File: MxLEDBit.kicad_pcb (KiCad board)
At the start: 2 copper layers, 94 x 91.4 mm, 355 parts, among them P11 CONN_01X01, P12 CONN_01X01, P13 CONN_01X01, P14 CONN_01X01, P15 CONN_01X01, P16 CONN_01X01, P2 CONN_01X01, P21 CONN_01X01, P22 CONN_01X01, P23 CONN_01X01, P24 CONN_01X01, SW1 SW_PUSH, U1 SK6812mini, U2 ProMicro

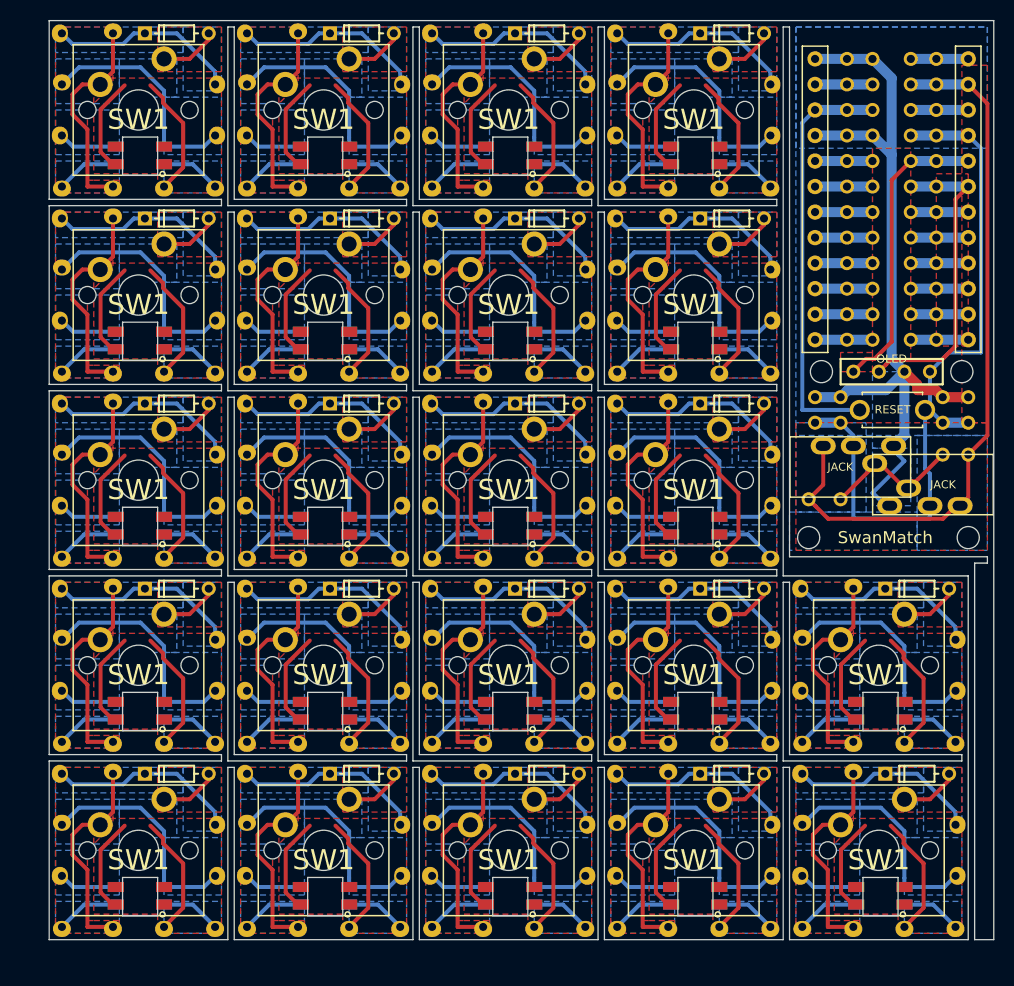
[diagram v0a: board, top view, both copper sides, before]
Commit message: second ordered
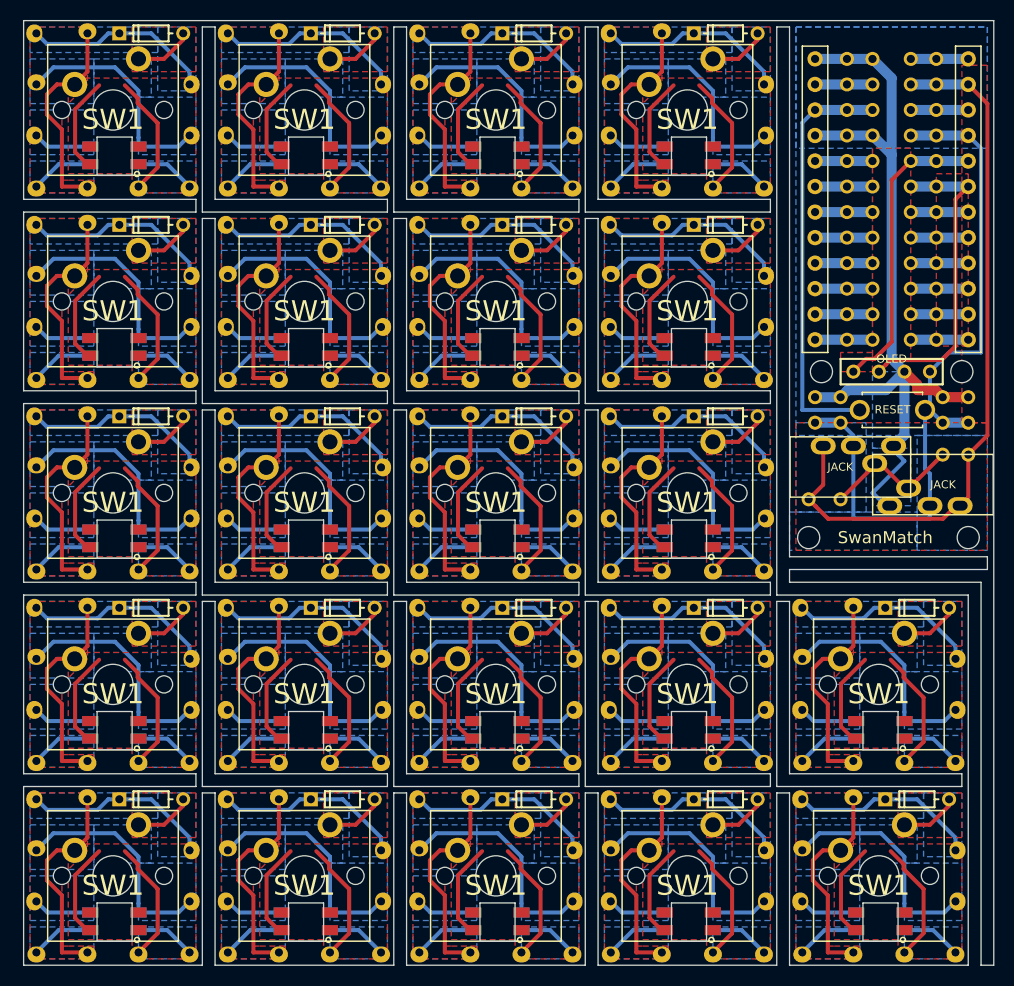
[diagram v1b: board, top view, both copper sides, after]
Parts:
- moved P11 3.59 mm to (85.7, 122.6)
- moved P12 3.59 mm to (80.6, 127.6)
- moved P23 3.59 mm to (80.6, 122.6)
- moved SW1 3.59 mm to (88.3, 130.2)
- moved D1 3.59 mm to (88.9, 122.6)
- moved P13 3.59 mm to (85.7, 137.8)
- moved P14 3.59 mm to (80.6, 137.8)
- moved P22 3.59 mm to (95.9, 127.6)
- moved P24 3.59 mm to (80.6, 132.7)
- moved P15 3.59 mm to (95.9, 137.8)
- moved P16 3.59 mm to (90.8, 137.8)
- moved P21 3.59 mm to (95.9, 132.7)
- moved U1 3.59 mm to (88.4, 134.7)
- moved D1 3.18 mm to (108.0, 122.6)
- moved P11 3.18 mm to (85.7, 103.5)
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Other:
- board size 94 x 91.4 mm -> 96.5 x 94 mm

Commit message: v2
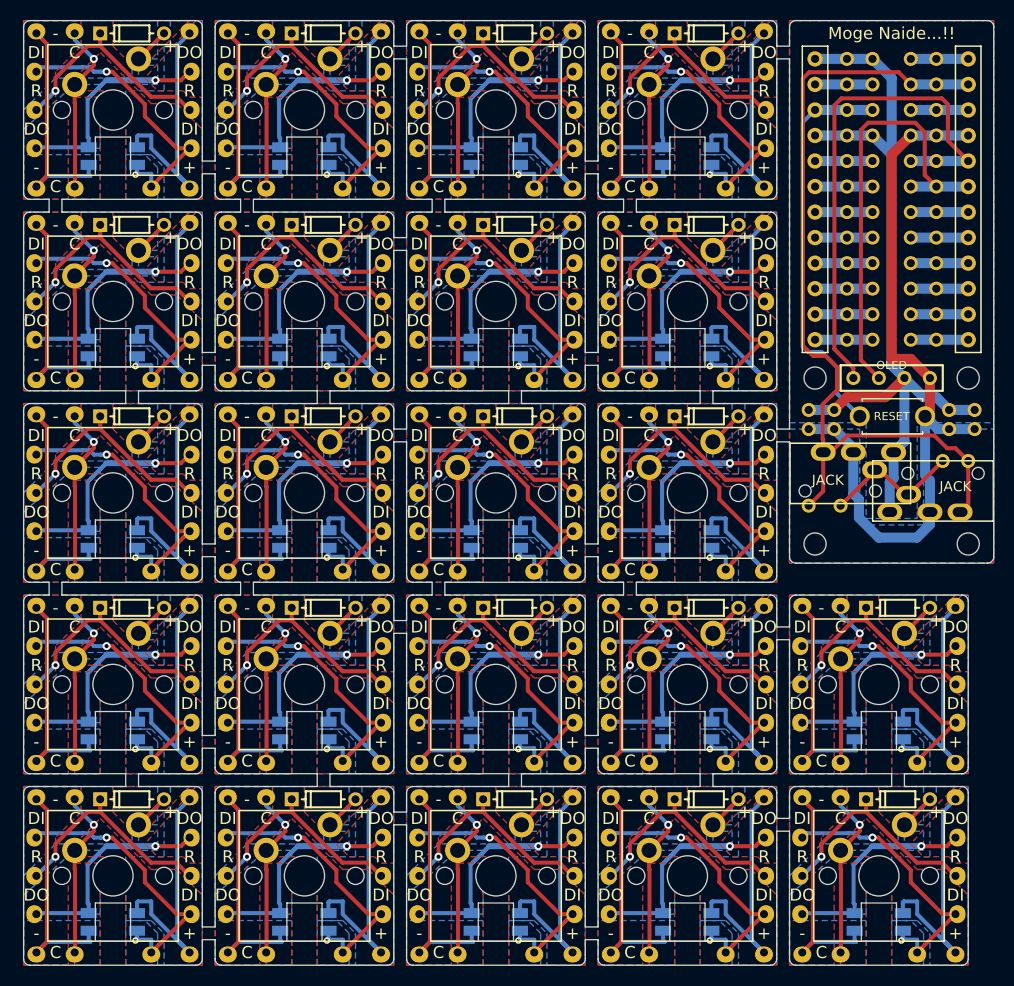
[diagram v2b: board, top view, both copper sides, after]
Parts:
- removed the D1 at (165.1, 122.6)
- removed the D1 at (88.9, 103.5)
- removed the D1 at (146.1, 84.5)
- removed the D1 at (127.0, 84.5)
- removed the D1 at (108.0, 84.5)
- removed the D1 at (88.9, 84.5)
- removed the D1 at (146.1, 65.4)
- removed the D1 at (127.0, 65.4)
- removed the D1 at (108.0, 65.4)
- removed the D1 at (88.9, 65.4)
- removed the D1 at (146.1, 46.4)
- removed the D1 at (165.1, 103.5)
- removed the D1 at (127.0, 46.4)
- removed the D1 at (108.0, 46.4)
- removed the D1 at (146.1, 122.6)
- removed the D1 at (127.0, 122.6)
- removed the D1 at (108.0, 122.6)
- removed the D1 at (88.9, 122.6)
- removed the D1 at (146.1, 103.5)
- removed the D1 at (127.0, 103.5)
- removed the D1 at (108.0, 103.5)
- removed the P11 at (161.9, 122.6)
- removed the P11 at (85.7, 103.5)
- removed the P11 at (142.9, 84.5)
- removed the P11 at (123.8, 84.5)
- removed the P11 at (104.8, 84.5)
- removed the P11 at (85.7, 84.5)
- removed the P11 at (142.9, 65.4)
- removed the P11 at (123.8, 65.4)
- removed the P11 at (104.8, 65.4)
- removed the P11 at (85.7, 65.4)
- removed the P11 at (142.9, 46.4)
- removed the P11 at (161.9, 103.5)
- removed the P11 at (123.8, 46.4)
- removed the P11 at (104.8, 46.4)
- removed the P11 at (142.9, 122.6)
- removed the P11 at (123.8, 122.6)
- removed the P11 at (104.8, 122.6)
- removed the P11 at (85.7, 122.6)
- removed the P11 at (142.9, 103.5)
- removed the P11 at (123.8, 103.5)
- removed the P11 at (104.8, 103.5)
- removed the P12 at (156.8, 127.6)
- removed the P12 at (80.6, 108.6)
- removed the P12 at (137.8, 89.5)
- removed the P12 at (118.7, 89.5)
- removed the P12 at (99.7, 89.5)
- removed the P12 at (80.6, 89.5)
- removed the P12 at (137.8, 70.5)
- removed the P12 at (118.7, 70.5)
- removed the P12 at (99.7, 70.5)
- removed the P12 at (80.6, 70.5)
- removed the P12 at (137.8, 51.4)
- removed the P12 at (156.8, 108.6)
- removed the P12 at (118.7, 51.4)
- removed the P12 at (99.7, 51.4)
- removed the P12 at (137.8, 127.6)
- removed the P12 at (118.7, 127.6)
- removed the P12 at (99.7, 127.6)
- removed the P12 at (80.6, 127.6)
- removed the P12 at (137.8, 108.6)
- removed the P12 at (118.7, 108.6)
- removed the P12 at (99.7, 108.6)
- removed P13 (x22), P14 (x22): CONN_01X01, footprint:wirepad
- removed the P16 at (167.0, 118.7)
- removed the P16 at (90.8, 118.7)
- removed the P16 at (148.0, 99.7)
- removed the P16 at (128.9, 99.7)
- removed the P16 at (109.9, 99.7)
- removed the P16 at (90.8, 99.7)
- removed the P16 at (148.0, 80.6)
- removed the P16 at (128.9, 80.6)
- removed the P16 at (109.9, 80.6)
- removed the P16 at (90.8, 80.6)
- removed the P16 at (148.0, 61.6)
- removed the P16 at (167.0, 137.8)
- removed the P16 at (128.9, 61.6)
- removed the P16 at (109.9, 61.6)
- removed the P16 at (148.0, 137.8)
- removed the P16 at (128.9, 137.8)
- removed the P16 at (109.9, 137.8)
- removed the P16 at (90.8, 137.8)
- removed the P16 at (148.0, 118.7)
- removed the P16 at (128.9, 118.7)
- removed the P16 at (109.9, 118.7)
- removed the P21 at (172.1, 113.7)
- removed the P21 at (95.9, 113.7)
- removed the P21 at (153.0, 94.6)
- removed the P21 at (134.0, 94.6)
- removed the P21 at (114.9, 94.6)
- removed the P21 at (95.9, 94.6)
- removed the P21 at (153.0, 75.6)
- removed the P21 at (134.0, 75.6)
- removed the P21 at (114.9, 75.6)
- removed the P21 at (95.9, 75.6)
- removed the P21 at (153.0, 56.5)
- removed the P21 at (172.1, 132.7)
- removed the P21 at (134.0, 56.5)
- removed the P21 at (114.9, 56.5)
- removed the P21 at (153.0, 132.7)
- removed the P21 at (134.0, 132.7)
- removed the P21 at (114.9, 132.7)
- removed the P21 at (95.9, 132.7)
- removed the P21 at (153.0, 113.7)
- removed the P21 at (134.0, 113.7)
- removed the P21 at (114.9, 113.7)
- removed the P22 at (172.1, 108.6)
- removed the P22 at (95.9, 108.6)
- removed the P22 at (153.0, 89.5)
- removed the P22 at (134.0, 89.5)
- removed the P22 at (114.9, 89.5)
- removed the P22 at (95.9, 89.5)
- removed the P22 at (153.0, 70.5)
- removed the P22 at (134.0, 70.5)
- removed the P22 at (114.9, 70.5)
- removed the P22 at (95.9, 70.5)
- removed the P22 at (153.0, 51.4)
- removed the P22 at (172.1, 127.6)
- removed the P22 at (134.0, 51.4)
- removed the P22 at (114.9, 51.4)
- removed the P22 at (95.9, 51.4)
- removed the P22 at (153.0, 127.6)
- removed the P22 at (134.0, 127.6)
- removed the P22 at (114.9, 127.6)
- removed the P22 at (95.9, 127.6)
- removed the P22 at (153.0, 108.6)
- removed the P22 at (134.0, 108.6)
- removed the P22 at (114.9, 108.6)
- removed the P24 at (156.8, 132.7)
- removed the P24 at (80.6, 113.7)
- removed the P24 at (137.8, 94.6)
- removed the P24 at (118.7, 94.6)
- removed the P24 at (99.7, 94.6)
- removed the P24 at (80.6, 94.6)
- removed the P24 at (137.8, 75.6)
- removed the P24 at (118.7, 75.6)
- removed the P24 at (99.7, 75.6)
- removed the P24 at (80.6, 75.6)
- removed the P24 at (137.8, 56.5)
- removed the P24 at (156.8, 113.7)
- removed the P24 at (118.7, 56.5)
- removed the P24 at (99.7, 56.5)
- removed the P24 at (137.8, 132.7)
- removed the P24 at (118.7, 132.7)
- removed the P24 at (99.7, 132.7)
- removed the P24 at (80.6, 132.7)
- removed the P24 at (137.8, 113.7)
- removed the P24 at (118.7, 113.7)
- removed the P24 at (99.7, 113.7)
- removed the U1 at (164.6, 115.6)
- removed the U1 at (88.4, 115.6)
- removed the U1 at (145.6, 96.6)
- removed the U1 at (126.5, 96.6)
- removed the U1 at (107.5, 96.6)
- removed the U1 at (88.4, 96.6)
- removed the U1 at (145.6, 77.5)
- removed the U1 at (126.5, 77.5)
- removed the U1 at (107.5, 77.5)
- removed the U1 at (88.4, 77.5)
- removed the U1 at (145.6, 58.5)
- removed the U1 at (164.6, 134.7)
- removed the U1 at (126.5, 58.5)
- removed the U1 at (107.5, 58.5)
- removed the U1 at (145.6, 134.7)
- removed the U1 at (126.5, 134.7)
- removed the U1 at (107.5, 134.7)
- removed the U1 at (88.4, 134.7)
- removed the U1 at (145.6, 115.6)
- removed the U1 at (126.5, 115.6)
- removed the U1 at (107.5, 115.6)
- added D1: D, footprint:diode, B.Cu at (163.2, 122.6)
- added D1: D, footprint:diode, B.Cu at (87.0, 103.5)
- added D1: D, footprint:diode, B.Cu at (144.1, 84.5)
- added D1: D, footprint:diode, B.Cu at (125.1, 84.5)
- added D1: D, footprint:diode, B.Cu at (106.0, 84.5)
- added D1: D, footprint:diode, B.Cu at (87.0, 84.5)
- added D1: D, footprint:diode, B.Cu at (144.1, 65.4)
- added D1: D, footprint:diode, B.Cu at (125.1, 65.4)
- added D1: D, footprint:diode, B.Cu at (106.0, 65.4)
- added D1: D, footprint:diode, B.Cu at (87.0, 65.4)
- added D1: D, footprint:diode, B.Cu at (144.1, 46.4)
- added D1: D, footprint:diode, B.Cu at (163.2, 103.5)
- added D1: D, footprint:diode, B.Cu at (125.1, 46.4)
- added D1: D, footprint:diode, B.Cu at (106.0, 46.4)
- added D1: D, footprint:diode, B.Cu at (144.1, 122.6)
- added D1: D, footprint:diode, B.Cu at (125.1, 122.6)
- added D1: D, footprint:diode, B.Cu at (106.0, 122.6)
- added D1: D, footprint:diode, B.Cu at (87.0, 122.6)
- added D1: D, footprint:diode, B.Cu at (144.1, 103.5)
- added D1: D, footprint:diode, B.Cu at (125.1, 103.5)
- added D1: D, footprint:diode, B.Cu at (106.0, 103.5)
- added P11: CONN_01X01, footprint:wirepad, F.Cu at (160.7, 103.5)
- added P11: CONN_01X01, footprint:wirepad, F.Cu at (122.6, 103.5)
- added P11: CONN_01X01, footprint:wirepad, F.Cu at (103.5, 103.5)
- added P11: CONN_01X01, footprint:wirepad, F.Cu at (84.5, 103.5)
- added P11: CONN_01X01, footprint:wirepad, F.Cu at (141.6, 84.5)
- added P11: CONN_01X01, footprint:wirepad, F.Cu at (122.6, 84.5)
- added P11: CONN_01X01, footprint:wirepad, F.Cu at (103.5, 84.5)
- added P11: CONN_01X01, footprint:wirepad, F.Cu at (84.5, 84.5)
- added P11: CONN_01X01, footprint:wirepad, F.Cu at (141.6, 65.4)
- added P11: CONN_01X01, footprint:wirepad, F.Cu at (122.6, 65.4)
- added P11: CONN_01X01, footprint:wirepad, F.Cu at (103.5, 65.4)
- added P11: CONN_01X01, footprint:wirepad, F.Cu at (160.7, 122.6)
- added P11: CONN_01X01, footprint:wirepad, F.Cu at (84.5, 65.4)
- added P11: CONN_01X01, footprint:wirepad, F.Cu at (141.6, 46.4)
- added P11: CONN_01X01, footprint:wirepad, F.Cu at (122.6, 46.4)
- added P11: CONN_01X01, footprint:wirepad, F.Cu at (103.5, 46.4)
- added P11: CONN_01X01, footprint:wirepad, F.Cu at (141.6, 137.8)
- added P11: CONN_01X01, footprint:wirepad, F.Cu at (122.6, 137.8)
- added P11: CONN_01X01, footprint:wirepad, F.Cu at (103.5, 137.8)
- added P11: CONN_01X01, footprint:wirepad, F.Cu at (84.5, 137.8)
- added P11: CONN_01X01, footprint:wirepad, F.Cu at (141.6, 118.7)
- added P11: CONN_01X01, footprint:wirepad, F.Cu at (122.6, 118.7)
- added P11: CONN_01X01, footprint:wirepad, F.Cu at (160.7, 118.7)
- added P11: CONN_01X01, footprint:wirepad, F.Cu at (103.5, 118.7)
- added P11: CONN_01X01, footprint:wirepad, F.Cu at (84.5, 118.7)
- added P11: CONN_01X01, footprint:wirepad, F.Cu at (141.6, 99.7)
- added P11: CONN_01X01, footprint:wirepad, F.Cu at (122.6, 99.7)
- added P11: CONN_01X01, footprint:wirepad, F.Cu at (103.5, 99.7)
- added P11: CONN_01X01, footprint:wirepad, F.Cu at (84.5, 99.7)
- added P11: CONN_01X01, footprint:wirepad, F.Cu at (141.6, 80.6)
- added P11: CONN_01X01, footprint:wirepad, F.Cu at (122.6, 80.6)
- added P11: CONN_01X01, footprint:wirepad, F.Cu at (103.5, 80.6)
- added P11: CONN_01X01, footprint:wirepad, F.Cu at (84.5, 80.6)
- added P11: CONN_01X01, footprint:wirepad, F.Cu at (160.7, 137.8)
- added P11: CONN_01X01, footprint:wirepad, F.Cu at (141.6, 61.6)
- added P11: CONN_01X01, footprint:wirepad, F.Cu at (122.6, 61.6)
- added P11: CONN_01X01, footprint:wirepad, F.Cu at (103.5, 61.6)
- added P11: CONN_01X01, footprint:wirepad, F.Cu at (84.5, 61.6)
- added P11: CONN_01X01, footprint:wirepad, F.Cu at (141.6, 122.6)
- added P11: CONN_01X01, footprint:wirepad, F.Cu at (122.6, 122.6)
- added P11: CONN_01X01, footprint:wirepad, F.Cu at (103.5, 122.6)
- added P11: CONN_01X01, footprint:wirepad, F.Cu at (84.5, 122.6)
- added P11: CONN_01X01, footprint:wirepad, F.Cu at (141.6, 103.5)
- added P12: CONN_01X01, footprint:wirepad, F.Cu at (156.8, 114.9)
- added P12: CONN_01X01, footprint:wirepad, F.Cu at (134.0, 107.3)
- added P12: CONN_01X01, footprint:wirepad, F.Cu at (114.9, 107.3)
- added P12: CONN_01X01, footprint:wirepad, F.Cu at (95.9, 107.3)
- added P12: CONN_01X01, footprint:wirepad, F.Cu at (153.0, 88.3)
- added P12: CONN_01X01, footprint:wirepad, F.Cu at (134.0, 88.3)
- added P12: CONN_01X01, footprint:wirepad, F.Cu at (114.9, 88.3)
- added P12: CONN_01X01, footprint:wirepad, F.Cu at (95.9, 88.3)
- added P12: CONN_01X01, footprint:wirepad, F.Cu at (153.0, 69.2)
- added P12: CONN_01X01, footprint:wirepad, F.Cu at (134.0, 69.2)
- added P12: CONN_01X01, footprint:wirepad, F.Cu at (114.9, 69.2)
- added P12: CONN_01X01, footprint:wirepad, F.Cu at (156.8, 134.0)
- added P12: CONN_01X01, footprint:wirepad, F.Cu at (95.9, 69.2)
- added P12: CONN_01X01, footprint:wirepad, F.Cu at (153.0, 50.2)
- added P12: CONN_01X01, footprint:wirepad, F.Cu at (134.0, 50.2)
- added P12: CONN_01X01, footprint:wirepad, F.Cu at (114.9, 50.2)
- added P12: CONN_01X01, footprint:wirepad, F.Cu at (137.8, 134.0)
- added P12: CONN_01X01, footprint:wirepad, F.Cu at (118.7, 134.0)
- added P12: CONN_01X01, footprint:wirepad, F.Cu at (99.7, 134.0)
- added P12: CONN_01X01, footprint:wirepad, F.Cu at (80.6, 134.0)
- added P12: CONN_01X01, footprint:wirepad, F.Cu at (137.8, 114.9)
- added P12: CONN_01X01, footprint:wirepad, F.Cu at (118.7, 114.9)
- added P12: CONN_01X01, footprint:wirepad, F.Cu at (172.1, 126.4)
- added P12: CONN_01X01, footprint:wirepad, F.Cu at (99.7, 114.9)
- added P12: CONN_01X01, footprint:wirepad, F.Cu at (80.6, 114.9)
- added P12: CONN_01X01, footprint:wirepad, F.Cu at (137.8, 95.9)
- added P12: CONN_01X01, footprint:wirepad, F.Cu at (118.7, 95.9)
- added P12: CONN_01X01, footprint:wirepad, F.Cu at (99.7, 95.9)
- added P12: CONN_01X01, footprint:wirepad, F.Cu at (80.6, 95.9)
- added P12: CONN_01X01, footprint:wirepad, F.Cu at (137.8, 76.8)
- added P12: CONN_01X01, footprint:wirepad, F.Cu at (118.7, 76.8)
- added P12: CONN_01X01, footprint:wirepad, F.Cu at (99.7, 76.8)
- added P12: CONN_01X01, footprint:wirepad, F.Cu at (80.6, 76.8)
- added P12: CONN_01X01, footprint:wirepad, F.Cu at (172.1, 107.3)
- added P12: CONN_01X01, footprint:wirepad, F.Cu at (137.8, 57.8)
- added P12: CONN_01X01, footprint:wirepad, F.Cu at (118.7, 57.8)
- added P12: CONN_01X01, footprint:wirepad, F.Cu at (99.7, 57.8)
- added P12: CONN_01X01, footprint:wirepad, F.Cu at (95.9, 50.2)
- added P12: CONN_01X01, footprint:wirepad, F.Cu at (153.0, 126.4)
- added P12: CONN_01X01, footprint:wirepad, F.Cu at (134.0, 126.4)
- added P12: CONN_01X01, footprint:wirepad, F.Cu at (114.9, 126.4)
- added P12: CONN_01X01, footprint:wirepad, F.Cu at (95.9, 126.4)
- added P12: CONN_01X01, footprint:wirepad, F.Cu at (153.0, 107.3)
- added P16: CONN_01X01, footprint:wirepad, F.Cu at (168.3, 118.7)
- added P16: CONN_01X01, footprint:wirepad, F.Cu at (92.1, 118.7)
- added P16: CONN_01X01, footprint:wirepad, F.Cu at (149.2, 99.7)
- added P16: CONN_01X01, footprint:wirepad, F.Cu at (130.2, 99.7)
- added P16: CONN_01X01, footprint:wirepad, F.Cu at (111.1, 99.7)
- added P16: CONN_01X01, footprint:wirepad, F.Cu at (92.1, 99.7)
- added P16: CONN_01X01, footprint:wirepad, F.Cu at (149.2, 80.6)
- added P16: CONN_01X01, footprint:wirepad, F.Cu at (130.2, 80.6)
- added P16: CONN_01X01, footprint:wirepad, F.Cu at (111.1, 80.6)
- added P16: CONN_01X01, footprint:wirepad, F.Cu at (92.1, 80.6)
- added P16: CONN_01X01, footprint:wirepad, F.Cu at (149.2, 61.6)
- added P16: CONN_01X01, footprint:wirepad, F.Cu at (168.3, 137.8)
- added P16: CONN_01X01, footprint:wirepad, F.Cu at (130.2, 61.6)
- added P16: CONN_01X01, footprint:wirepad, F.Cu at (111.1, 61.6)
- added P16: CONN_01X01, footprint:wirepad, F.Cu at (149.2, 137.8)
- added P16: CONN_01X01, footprint:wirepad, F.Cu at (130.2, 137.8)
- added P16: CONN_01X01, footprint:wirepad, F.Cu at (111.1, 137.8)
- added P16: CONN_01X01, footprint:wirepad, F.Cu at (92.1, 137.8)
- added P16: CONN_01X01, footprint:wirepad, F.Cu at (149.2, 118.7)
- added P16: CONN_01X01, footprint:wirepad, F.Cu at (130.2, 118.7)
- added P16: CONN_01X01, footprint:wirepad, F.Cu at (111.1, 118.7)
- added P21: CONN_01X01, footprint:wirepad, F.Cu at (172.1, 134.0)
- added P21: CONN_01X01, footprint:wirepad, F.Cu at (95.9, 114.9)
- added P21: CONN_01X01, footprint:wirepad, F.Cu at (153.0, 95.9)
- added P21: CONN_01X01, footprint:wirepad, F.Cu at (134.0, 95.9)
- added P21: CONN_01X01, footprint:wirepad, F.Cu at (114.9, 95.9)
- added P21: CONN_01X01, footprint:wirepad, F.Cu at (95.9, 95.9)
- added P21: CONN_01X01, footprint:wirepad, F.Cu at (153.0, 76.8)
- added P21: CONN_01X01, footprint:wirepad, F.Cu at (134.0, 76.8)
- added P21: CONN_01X01, footprint:wirepad, F.Cu at (114.9, 76.8)
- added P21: CONN_01X01, footprint:wirepad, F.Cu at (95.9, 76.8)
- added P21: CONN_01X01, footprint:wirepad, F.Cu at (153.0, 57.8)
- added P21: CONN_01X01, footprint:wirepad, F.Cu at (172.1, 114.9)
- added P21: CONN_01X01, footprint:wirepad, F.Cu at (134.0, 57.8)
- added P21: CONN_01X01, footprint:wirepad, F.Cu at (114.9, 57.8)
- added P21: CONN_01X01, footprint:wirepad, F.Cu at (153.0, 134.0)
- added P21: CONN_01X01, footprint:wirepad, F.Cu at (134.0, 134.0)
- added P21: CONN_01X01, footprint:wirepad, F.Cu at (114.9, 134.0)
- added P21: CONN_01X01, footprint:wirepad, F.Cu at (95.9, 134.0)
- added P21: CONN_01X01, footprint:wirepad, F.Cu at (153.0, 114.9)
- added P21: CONN_01X01, footprint:wirepad, F.Cu at (134.0, 114.9)
- added P21: CONN_01X01, footprint:wirepad, F.Cu at (114.9, 114.9)
- added P22: CONN_01X01, footprint:wirepad, F.Cu at (172.1, 130.2)
- added P22: CONN_01X01, footprint:wirepad, F.Cu at (95.9, 111.1)
- added P22: CONN_01X01, footprint:wirepad, F.Cu at (153.0, 92.1)
- added P22: CONN_01X01, footprint:wirepad, F.Cu at (134.0, 92.1)
- added P22: CONN_01X01, footprint:wirepad, F.Cu at (114.9, 92.1)
- added P22: CONN_01X01, footprint:wirepad, F.Cu at (95.9, 92.1)
- added P22: CONN_01X01, footprint:wirepad, F.Cu at (153.0, 73.0)
- added P22: CONN_01X01, footprint:wirepad, F.Cu at (134.0, 73.0)
- added P22: CONN_01X01, footprint:wirepad, F.Cu at (114.9, 73.0)
- added P22: CONN_01X01, footprint:wirepad, F.Cu at (95.9, 73.0)
- added P22: CONN_01X01, footprint:wirepad, F.Cu at (153.0, 54.0)
- added P22: CONN_01X01, footprint:wirepad, F.Cu at (172.1, 111.1)
- added P22: CONN_01X01, footprint:wirepad, F.Cu at (134.0, 54.0)
- added P22: CONN_01X01, footprint:wirepad, F.Cu at (114.9, 54.0)
- added P22: CONN_01X01, footprint:wirepad, F.Cu at (95.9, 54.0)
- added P22: CONN_01X01, footprint:wirepad, F.Cu at (153.0, 130.2)
- added P22: CONN_01X01, footprint:wirepad, F.Cu at (134.0, 130.2)
- added P22: CONN_01X01, footprint:wirepad, F.Cu at (114.9, 130.2)
- added P22: CONN_01X01, footprint:wirepad, F.Cu at (95.9, 130.2)
- added P22: CONN_01X01, footprint:wirepad, F.Cu at (153.0, 111.1)
- added P22: CONN_01X01, footprint:wirepad, F.Cu at (134.0, 111.1)
- added P22: CONN_01X01, footprint:wirepad, F.Cu at (114.9, 111.1)
- added P23: CONN_01X01, footprint:wirepad, F.Cu at (172.1, 122.6)
- added P23: CONN_01X01, footprint:wirepad, F.Cu at (118.7, 137.8)
- added P23: CONN_01X01, footprint:wirepad, F.Cu at (99.7, 137.8)
- added P23: CONN_01X01, footprint:wirepad, F.Cu at (80.6, 137.8)
- added P23: CONN_01X01, footprint:wirepad, F.Cu at (137.8, 118.7)
- added P23: CONN_01X01, footprint:wirepad, F.Cu at (118.7, 118.7)
- added P23: CONN_01X01, footprint:wirepad, F.Cu at (99.7, 118.7)
- added P23: CONN_01X01, footprint:wirepad, F.Cu at (80.6, 118.7)
- added P23: CONN_01X01, footprint:wirepad, F.Cu at (137.8, 99.7)
- added P23: CONN_01X01, footprint:wirepad, F.Cu at (118.7, 99.7)
- added P23: CONN_01X01, footprint:wirepad, F.Cu at (99.7, 99.7)
- added P23: CONN_01X01, footprint:wirepad, F.Cu at (156.8, 111.1)
- added P23: CONN_01X01, footprint:wirepad, F.Cu at (80.6, 99.7)
- added P23: CONN_01X01, footprint:wirepad, F.Cu at (137.8, 80.6)
- added P23: CONN_01X01, footprint:wirepad, F.Cu at (118.7, 80.6)
- added P23: CONN_01X01, footprint:wirepad, F.Cu at (99.7, 80.6)
- added P23: CONN_01X01, footprint:wirepad, F.Cu at (80.6, 80.6)
- added P23: CONN_01X01, footprint:wirepad, F.Cu at (137.8, 61.6)
- added P23: CONN_01X01, footprint:wirepad, F.Cu at (118.7, 61.6)
- added P23: CONN_01X01, footprint:wirepad, F.Cu at (99.7, 61.6)
- added P23: CONN_01X01, footprint:wirepad, F.Cu at (172.1, 103.5)
- added P23: CONN_01X01, footprint:wirepad, F.Cu at (137.8, 130.2)
- added P23: CONN_01X01, footprint:wirepad, F.Cu at (118.7, 130.2)
- added P23: CONN_01X01, footprint:wirepad, F.Cu at (99.7, 130.2)
- added P23: CONN_01X01, footprint:wirepad, F.Cu at (156.8, 137.8)
- added P23: CONN_01X01, footprint:wirepad, F.Cu at (80.6, 130.2)
- added P23: CONN_01X01, footprint:wirepad, F.Cu at (137.8, 111.1)
- added P23: CONN_01X01, footprint:wirepad, F.Cu at (118.7, 111.1)
- added P23: CONN_01X01, footprint:wirepad, F.Cu at (99.7, 111.1)
- added P23: CONN_01X01, footprint:wirepad, F.Cu at (80.6, 111.1)
- added P23: CONN_01X01, footprint:wirepad, F.Cu at (137.8, 92.1)
- added P23: CONN_01X01, footprint:wirepad, F.Cu at (118.7, 92.1)
- added P23: CONN_01X01, footprint:wirepad, F.Cu at (99.7, 92.1)
- added P23: CONN_01X01, footprint:wirepad, F.Cu at (80.6, 92.1)
- added P23: CONN_01X01, footprint:wirepad, F.Cu at (137.8, 73.0)
- added P23: CONN_01X01, footprint:wirepad, F.Cu at (156.8, 118.7)
- added P23: CONN_01X01, footprint:wirepad, F.Cu at (118.7, 73.0)
- added P23: CONN_01X01, footprint:wirepad, F.Cu at (99.7, 73.0)
- added P23: CONN_01X01, footprint:wirepad, F.Cu at (80.6, 73.0)
- added P23: CONN_01X01, footprint:wirepad, F.Cu at (137.8, 54.0)
- added P23: CONN_01X01, footprint:wirepad, F.Cu at (118.7, 54.0)
- added P23: CONN_01X01, footprint:wirepad, F.Cu at (99.7, 54.0)
- added P23: CONN_01X01, footprint:wirepad, F.Cu at (153.0, 122.6)
- added P23: CONN_01X01, footprint:wirepad, F.Cu at (134.0, 122.6)
- added P23: CONN_01X01, footprint:wirepad, F.Cu at (114.9, 122.6)
- added P23: CONN_01X01, footprint:wirepad, F.Cu at (95.9, 122.6)
- added P23: CONN_01X01, footprint:wirepad, F.Cu at (153.0, 103.5)
- added P23: CONN_01X01, footprint:wirepad, F.Cu at (134.0, 103.5)
- added P23: CONN_01X01, footprint:wirepad, F.Cu at (114.9, 103.5)
- added P23: CONN_01X01, footprint:wirepad, F.Cu at (95.9, 103.5)
- added P23: CONN_01X01, footprint:wirepad, F.Cu at (153.0, 84.5)
- added P23: CONN_01X01, footprint:wirepad, F.Cu at (134.0, 84.5)
- added P23: CONN_01X01, footprint:wirepad, F.Cu at (114.9, 84.5)
- added P23: CONN_01X01, footprint:wirepad, F.Cu at (95.9, 84.5)
- added P23: CONN_01X01, footprint:wirepad, F.Cu at (153.0, 65.4)
- added P23: CONN_01X01, footprint:wirepad, F.Cu at (134.0, 65.4)
- added P23: CONN_01X01, footprint:wirepad, F.Cu at (156.8, 130.2)
- added P23: CONN_01X01, footprint:wirepad, F.Cu at (114.9, 65.4)
- added P23: CONN_01X01, footprint:wirepad, F.Cu at (95.9, 65.4)
- added P23: CONN_01X01, footprint:wirepad, F.Cu at (153.0, 46.4)
- added P23: CONN_01X01, footprint:wirepad, F.Cu at (134.0, 46.4)
- added P23: CONN_01X01, footprint:wirepad, F.Cu at (114.9, 46.4)
- added P23: CONN_01X01, footprint:wirepad, F.Cu at (80.6, 54.0)
- added P23: CONN_01X01, footprint:wirepad, F.Cu at (80.6, 61.6)
- added P23: CONN_01X01, footprint:wirepad, F.Cu at (80.6, 46.4)
- added P23: CONN_01X01, footprint:wirepad, F.Cu at (137.8, 137.8)
- added P24: CONN_01X01, footprint:wirepad, F.Cu at (156.8, 107.3)
- added P24: CONN_01X01, footprint:wirepad, F.Cu at (80.6, 107.3)
- added P24: CONN_01X01, footprint:wirepad, F.Cu at (137.8, 88.3)
- added P24: CONN_01X01, footprint:wirepad, F.Cu at (118.7, 88.3)
- added P24: CONN_01X01, footprint:wirepad, F.Cu at (99.7, 88.3)
- added P24: CONN_01X01, footprint:wirepad, F.Cu at (80.6, 88.3)
- added P24: CONN_01X01, footprint:wirepad, F.Cu at (137.8, 69.2)
- added P24: CONN_01X01, footprint:wirepad, F.Cu at (118.7, 69.2)
- added P24: CONN_01X01, footprint:wirepad, F.Cu at (99.7, 69.2)
- added P24: CONN_01X01, footprint:wirepad, F.Cu at (80.6, 69.2)
- added P24: CONN_01X01, footprint:wirepad, F.Cu at (137.8, 50.2)
- added P24: CONN_01X01, footprint:wirepad, F.Cu at (156.8, 126.4)
- added P24: CONN_01X01, footprint:wirepad, F.Cu at (118.7, 50.2)
- added P24: CONN_01X01, footprint:wirepad, F.Cu at (99.7, 50.2)
- added P24: CONN_01X01, footprint:wirepad, F.Cu at (137.8, 126.4)
- added P24: CONN_01X01, footprint:wirepad, F.Cu at (118.7, 126.4)
- added P24: CONN_01X01, footprint:wirepad, F.Cu at (99.7, 126.4)
- added P24: CONN_01X01, footprint:wirepad, F.Cu at (80.6, 126.4)
- added P24: CONN_01X01, footprint:wirepad, F.Cu at (137.8, 107.3)
- added P24: CONN_01X01, footprint:wirepad, F.Cu at (118.7, 107.3)
- added P24: CONN_01X01, footprint:wirepad, F.Cu at (99.7, 107.3)
- added U1: SK6812mini, sk6812:SK6812MINI_rev, F.Cu at (164.5, 134.8)
- added U1: SK6812mini, sk6812:SK6812MINI_rev, F.Cu at (88.3, 115.7)
- added U1: SK6812mini, sk6812:SK6812MINI_rev, F.Cu at (145.4, 96.7)
- added U1: SK6812mini, sk6812:SK6812MINI_rev, F.Cu at (126.4, 96.7)
- added U1: SK6812mini, sk6812:SK6812MINI_rev, F.Cu at (107.3, 96.7)
- added U1: SK6812mini, sk6812:SK6812MINI_rev, F.Cu at (88.3, 96.7)
- added U1: SK6812mini, sk6812:SK6812MINI_rev, F.Cu at (145.4, 77.6)
- added U1: SK6812mini, sk6812:SK6812MINI_rev, F.Cu at (126.4, 77.6)
- added U1: SK6812mini, sk6812:SK6812MINI_rev, F.Cu at (107.3, 77.6)
- added U1: SK6812mini, sk6812:SK6812MINI_rev, F.Cu at (88.3, 77.6)
- added U1: SK6812mini, sk6812:SK6812MINI_rev, F.Cu at (145.4, 58.6)
- added U1: SK6812mini, sk6812:SK6812MINI_rev, F.Cu at (164.5, 115.7)
- added U1: SK6812mini, sk6812:SK6812MINI_rev, F.Cu at (126.4, 58.6)
- added U1: SK6812mini, sk6812:SK6812MINI_rev, F.Cu at (107.3, 58.6)
- added U1: SK6812mini, sk6812:SK6812MINI_rev, F.Cu at (145.4, 134.8)
- added U1: SK6812mini, sk6812:SK6812MINI_rev, F.Cu at (126.4, 134.8)
- added U1: SK6812mini, sk6812:SK6812MINI_rev, F.Cu at (107.3, 134.8)
- added U1: SK6812mini, sk6812:SK6812MINI_rev, F.Cu at (88.3, 134.8)
- added U1: SK6812mini, sk6812:SK6812MINI_rev, F.Cu at (145.4, 115.7)
- added U1: SK6812mini, sk6812:SK6812MINI_rev, F.Cu at (126.4, 115.7)
- added U1: SK6812mini, sk6812:SK6812MINI_rev, F.Cu at (107.3, 115.7)
- JACK (x2): footprint MYLIB_REV:MJ-4PP-9_rev2 -> helix:MJ-4PP-9_rev2
- moved P23 15.2 mm to (95.9, 46.4), turned to 180 degrees
- moved P24 6.35 mm to (80.6, 50.2)
- moved P12 6.35 mm to (80.6, 57.8), turned to 270 degrees
- moved D1 1.91 mm to (87.0, 46.4)
- moved P2 1.42 mm to (174.0, 83.8)
- moved P2 1.42 mm to (157.5, 83.8)
- moved P2 1.42 mm to (171.4, 83.8)
- moved P2 1.42 mm to (160.0, 83.8)
- moved P11 1.27 mm to (84.5, 46.4)
- moved P16 1.27 mm to (92.1, 61.6)
- moved P21 1.27 mm to (95.9, 57.8)
- moved HOLE_M2 0.90 mm to (158.1, 97.2)
- moved P2 0.90 mm to (174.0, 85.7)
- moved P2 0.90 mm to (157.5, 85.7)
- moved HOLE_M2 0.90 mm to (173.4, 80.6)
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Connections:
- JACK pad B: VCC -> DATA (x2)
- JACK pad D: DATA -> VCC (x2)
- P12 pad 1: Net-(U1-Pad3) -> Net-(U1-Pad1)
- P15 pad 1: Net-(U1-Pad4) -> VCC (x22)
- P16 pad 1: Net-(U1-Pad2) -> Net-(U1-Pad4)
- P21 pad 1: Net-(U1-Pad3) -> Net-(U1-Pad4)
- P23 pad 1: /2 -> GND (x21)
- P23 pad 1: /2 -> VCC
- P24 pad 1: Net-(U1-Pad1) -> Net-(U1-Pad4)
- U1 pad 2: Net-(U1-Pad2) -> GND
- U1 pad 3: Net-(U1-Pad3) -> VCC
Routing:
- net Net-(U1-Pad2): track 619.1 -> 0.00 mm
- net VCC: track 81.4 -> 675.0 mm
- net GND: track 85.2 -> 595.0 mm
- net Net-(U1-Pad3): track 504.4 -> 0.00 mm
- net Net-(U1-Pad4): track 132.0 -> 623.9 mm, vias 0 -> 22
- net Net-(U1-Pad1): track 128.0 -> 525.5 mm, vias 0 -> 22
- net /1: track 478.1 -> 384.7 mm, vias 0 -> 22
- net /2: track 417.1 -> 495.3 mm, vias 0 -> 22
- net Net-(D1-Pad2): track 129.1 -> 79.0 mm
- net (no net): track 47.9 -> 13.6 mm
- net SDA: track 29.5 -> 51.9 mm
- net SCL: track 30.8 -> 44.1 mm
- net DATA: track 71.9 -> 85.1 mm
- net Net-(PM9-Pad1): track 0.00 -> 5.72 mm
- net Net-(PM8-Pad1): track 0.00 -> 5.72 mm
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- added copper zone on F.Cu, net GND
- added copper zone on F.Cu, net Net-(U1-Pad1)
- added copper zone on F.Cu, net Net-(U1-Pad4)
- removed copper zone on B.Cu, net /2
- removed copper zone on F.Cu, net DATA
- removed copper zone on B.Cu, net Net-(U1-Pad2)
- removed copper zone on F.Cu, net Net-(U1-Pad2)
- removed copper zone on B.Cu, net Net-(U1-Pad3)
- removed copper zone on F.Cu, net SCL
- removed copper zone on F.Cu, net SDA
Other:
- outline, holes or cut-outs redrawn
- net class GND added: clearance 0.254, trace_width 1, via_dia 0.8, via_drill 0.4
- board text added: "Moge Naide...!!"
- board text added: "OLED"
- board text added: "RESET"
